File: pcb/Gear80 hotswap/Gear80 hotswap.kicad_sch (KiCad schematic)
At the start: 206 parts, among them J3 Conn_01x04, U1 RP2040, U3 W25Q128JVSIQ, U4 XC6206P332MR, Y1 X322512MSB4SI

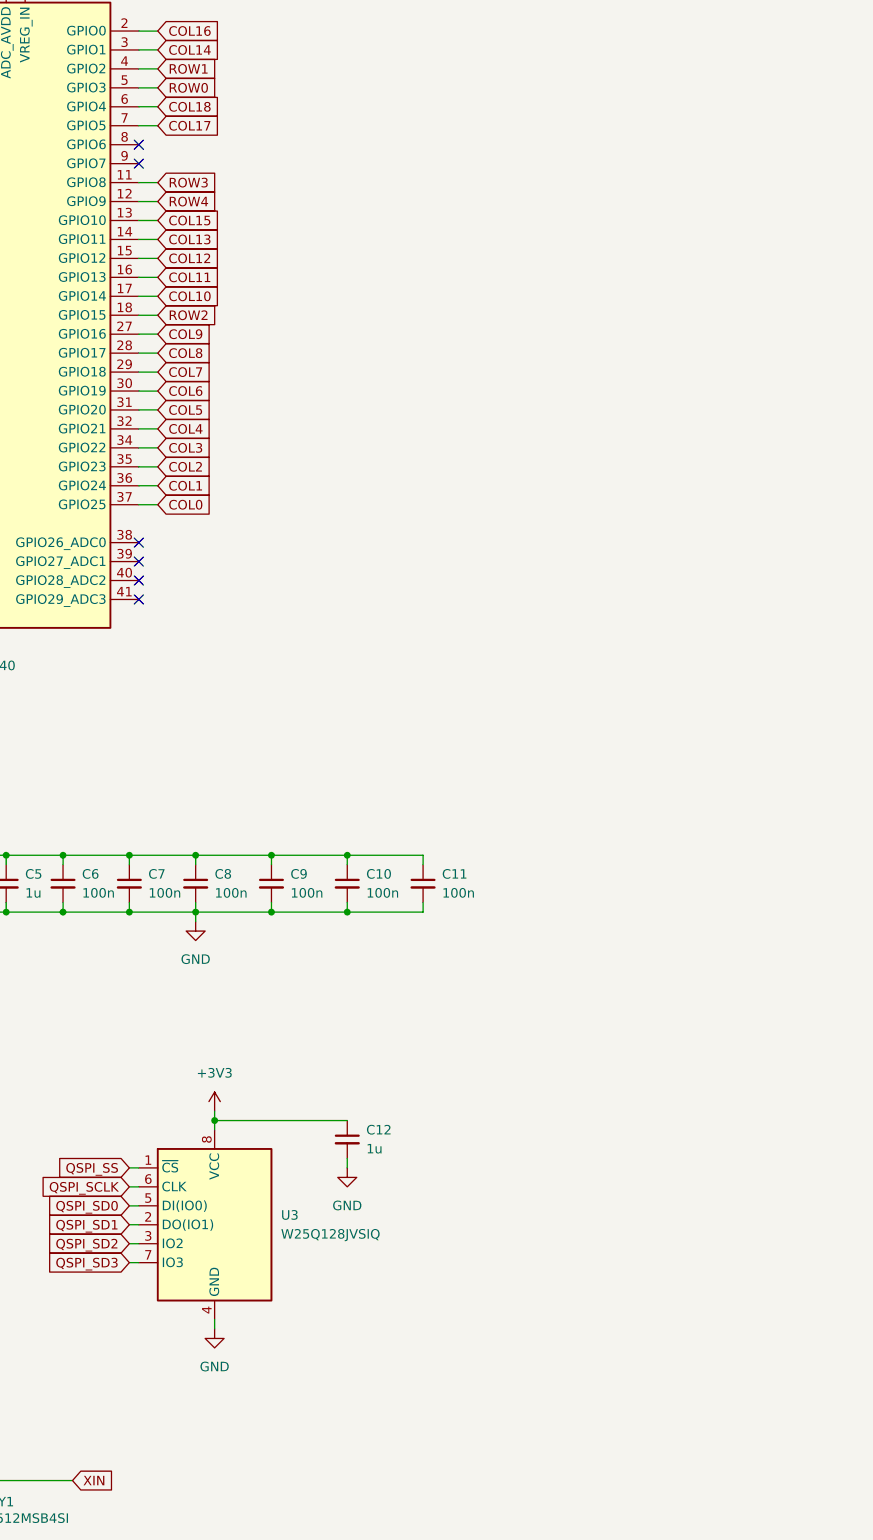
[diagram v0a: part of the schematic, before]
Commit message: Add files via upload
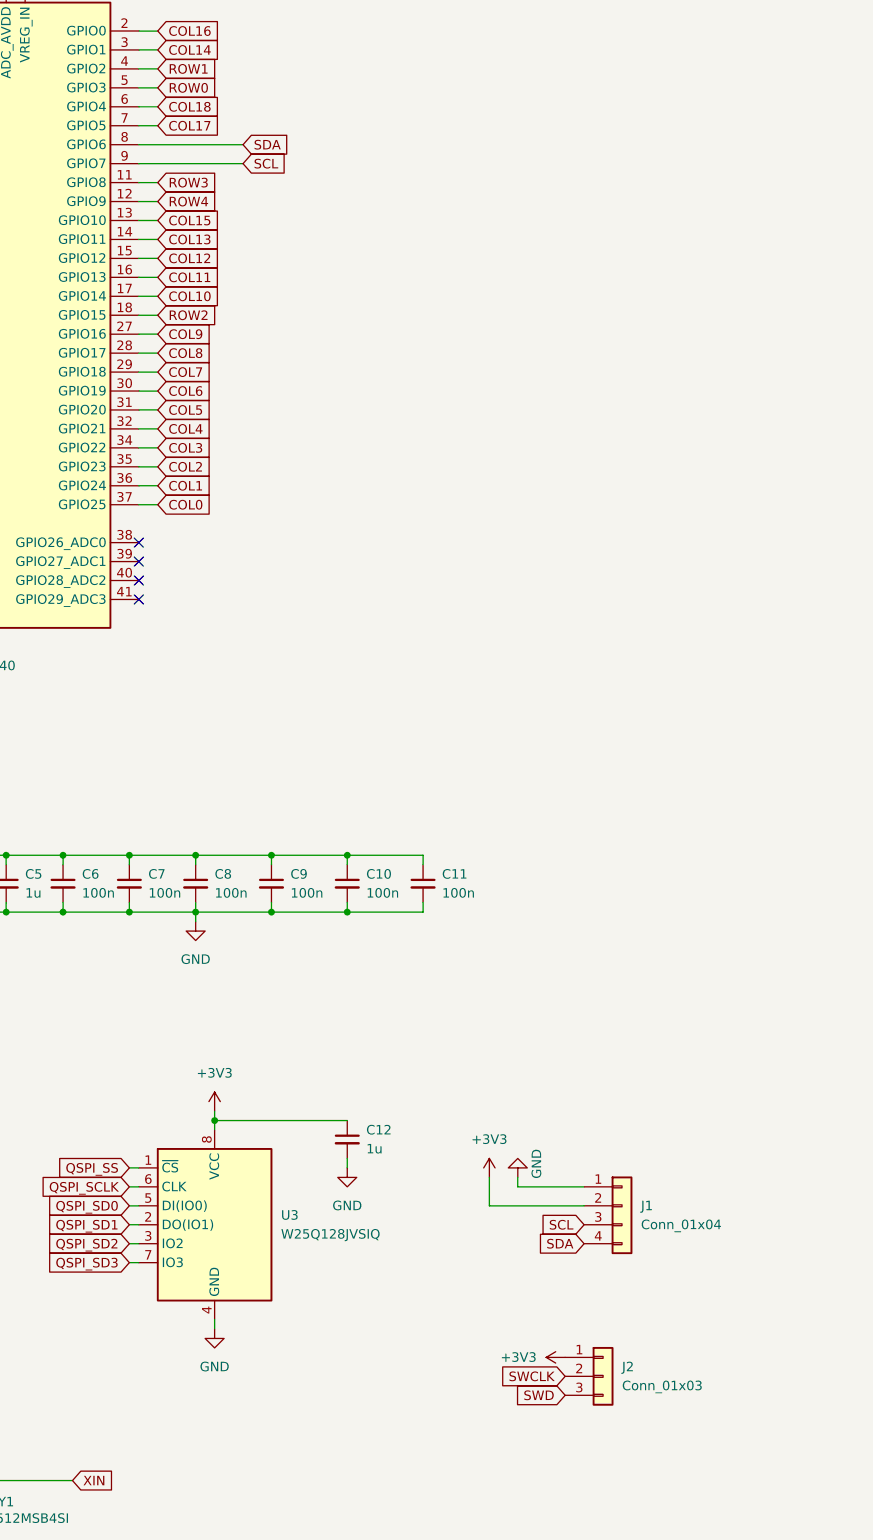
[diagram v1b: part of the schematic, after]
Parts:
- added J1: Conn_01x04, Connector_PinHeader_2.54mm:PinHeader_1x04_P2.54mm_Vertical, symbol Connector_Generic:Conn_01x04
- added J2: Conn_01x03, Connector_PinHeader_2.54mm:PinHeader_1x03_P2.54mm_Vertical, symbol Connector_Generic:Conn_01x03
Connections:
- net +3V3: now also J1.2 (Pin_2), J2.1 (Pin_1)
- net GND: now also J1.1 (Pin_1)
- net SWCLK: now also J2.2 (Pin_2)
- net SWD: now also J2.3 (Pin_3)
- net SDA: now reaches U1.8 (GPIO6)
- net SDA: now also J1.4 (Pin_4)
- net SCL: now reaches U1.9 (GPIO7)
- net SCL: now also J1.3 (Pin_3)
- no-connect marks 6 -> 4
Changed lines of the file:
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@@
   (no_connect (at 90.17 102.87))
   (no_connect (at 90.17 105.41))
-  (no_connect (at 90.17 49.53))
   (no_connect (at 90.17 107.95))
-  (no_connect (at 90.17 46.99))
   (no_connect (at 90.17 100.33))
   (wire (pts (xy 227.33 58.42) (xy 227.33 59.69))
@@
     (stroke (width 0) (type default))
   )
+  (wire (pts (xy 140.97 186.69) (xy 149.86 186.69))
+    (stroke (width 0) (type default))
+  )
   (wire (pts (xy 54.61 264.16) (xy 54.61 265.43))
     (stroke (width 0) (type default))
@@
     (stroke (width 0) (type default))
   )
+  (wire (pts (xy 137.16 189.23) (xy 137.16 185.42))
+    (stroke (width 0) (type default))
+  )
   (wire (pts (xy 327.66 64.77) (xy 342.9 64.77))
     (stroke (width 0) (type default))
@@
     (stroke (width 0) (type default))
   )
+  (wire (pts (xy 137.16 189.23) (xy 149.86 189.23))
+    (stroke (width 0) (type default))
+  )
   (wire (pts (xy 353.06 45.72) (xy 353.06 53.34))
     (stroke (width 0) (type default))
@@
     (stroke (width 0) (type default))
   )
+  (wire (pts (xy 104.14 46.99) (xy 90.17 46.99))
+    (stroke (width 0) (type default))
+  )
   (wire (pts (xy 227.33 64.77) (xy 269.24 64.77))
     (stroke (width 0) (type default))
@@
     (stroke (width 0) (type default))
   )
+  (wire (pts (xy 104.14 49.53) (xy 90.17 49.53))
+    (stroke (width 0) (type default))
+  )
   (wire (pts (xy 403.86 111.76) (xy 417.83 111.76))
     (stroke (width 0) (type default))
@@
     (stroke (width 0) (type default))
   )
+  (wire (pts (xy 140.97 185.42) (xy 140.97 186.69))
+    (stroke (width 0) (type default))
+  )
   (wire (pts (xy 398.78 124.46) (xy 398.78 147.32))
     (stroke (width 0) (type default))
@@
     )
   )
+  (global_label "SCL" (shape input) (at 104.14 49.53 0) (fields_autoplaced)
+    (effects (font (size 1.27 1.27)) (justify left))
+    (property "Intersheetrefs" "${INTERSHEET_REFS}" (at 110.6328 49.53 0)
+      (effects (font (size 1.27 1.27)) (justify left) hide)
+    )
+  )
   (global_label "QSPI_SS" (shape input) (at 55.88 278.13 0) (fields_autoplaced)
     (effects (font (size 1.27 1.27)) (justify left))
@@
     )
   )
+  (global_label "SDA" (shape input) (at 149.86 194.31 180) (fields_autoplaced)
+    (effects (font (size 1.27 1.27)) (justify right))
+    (property "Intersheetrefs" "${INTERSHEET_REFS}" (at 143.3067 194.31 0)
+      (effects (font (size 1.27 1.27)) (justify right) hide)
+    )
+  )
   (global_label "COL7" (shape input) (at 337.82 45.72 90) (fields_autoplaced)
     (effects (font (size 1.27 1.27)) (justify left))
@@
     )
   )
+  (global_label "SWD" (shape input) (at 147.32 214.63 180) (fields_autoplaced)
+    (effects (font (size 1.27 1.27)) (justify right))
+    (property "Intersheetrefs" "${INTERSHEET_REFS}" (at 140.4039 214.63 0)
+      (effects (font (size 1.27 1.27)) (justify right) hide)
+    )
+  )
   (global_label "COL0" (shape input) (at 92.71 95.25 0) (fields_autoplaced)
     (effects (font (size 1.27 1.27)) (justify left))
@@
     )
   )
+  (global_label "SWCLK" (shape input) (at 147.32 212.09 180) (fields_autoplaced)
+    (effects (font (size 1.27 1.27)) (justify right))
+    (property "Intersheetrefs" "${INTERSHEET_REFS}" (at 138.1058 212.09 0)
+      (effects (font (size 1.27 1.27)) (justify right) hide)
+    )
+  )
   (global_label "QSPI_SD1" (shape input) (at 88.9 191.77 180) (fields_autoplaced)
     (effects (font (size 1.27 1.27)) (justify right))
@@
     )
   )
+  (global_label "SDA" (shape input) (at 104.14 46.99 0) (fields_autoplaced)
+    (effects (font (size 1.27 1.27)) (justify left))
+    (property "Intersheetrefs" "${INTERSHEET_REFS}" (at 110.6933 46.99 0)
+      (effects (font (size 1.27 1.27)) (justify left) hide)
+    )
+  )
   (global_label "COL0" (shape input) (at 207.01 45.72 90) (fields_autoplaced)
     (effects (font (size 1.27 1.27)) (justify left))
@@
     )
   )
+  (global_label "SCL" (shape input) (at 149.86 191.77 180) (fields_autoplaced)
+    (effects (font (size 1.27 1.27)) (justify right))
+    (property "Intersheetrefs" "${INTERSHEET_REFS}" (at 143.3672 191.77 0)
+      (effects (font (size 1.27 1.27)) (justify right) hide)
+    )
+  )
   (global_label "XOUT" (shape input) (at 81.28 236.22 0) (fields_autoplaced)
     (effects (font (size 1.27 1.27)) (justify left))
@@
     )
   )
+  (symbol (lib_id "Connector_Generic:Conn_01x04") (at 154.94 189.23 0) (unit 1)
+    (in_bom yes) (on_board yes) (dnp no) (fields_autoplaced)
+    (property "Reference" "J1" (at 157.48 189.23 0)
+      (effects (font (size 1.27 1.27)) (justify left))
+    )
+    (property "Value" "Conn_01x04" (at 157.48 191.77 0)
+      (effects (font (size 1.27 1.27)) (justify left))
+    )
+    (property "Footprint" "Connector_PinHeader_2.54mm:PinHeader_1x04_P2.54mm_Vertical" (at 154.94 189.23 0)
+      (effects (font (size 1.27 1.27)) hide)
+    )
+    (property "Datasheet" "~" (at 154.94 189.23 0)
+      (effects (font (size 1.27 1.27)) hide)
+    )
+    (pin "1")
+    (pin "2")
+    (pin "3")
+    (pin "4")
+    (instances
+      (project "Gear80 hotswap"
+        (path "/3cbd346f-f2f7-49f7-a092-ced5397d72c6"
+          (reference "J1") (unit 1)
+        )
+      )
+    )
+  )
   (symbol (lib_id "power:GND") (at 118.11 184.15 0) (unit 1)
     (in_bom yes) (on_board yes) (dnp no) (fields_autoplaced)
@@
     )
   )
+  (symbol (lib_id "power:+3V3") (at 137.16 185.42 0) (unit 1)
+    (in_bom yes) (on_board yes) (dnp no) (fields_autoplaced)
+    (property "Reference" "#PWR08" (at 137.16 189.23 0)
+      (effects (font (size 1.27 1.27)) hide)
+    )
+    (property "Value" "+3V3" (at 137.16 180.34 0)
+      (effects (font (size 1.27 1.27)))
+    )
+    (property "Footprint" "" (at 137.16 185.42 0)
+      (effects (font (size 1.27 1.27)) hide)
+    )
+    (property "Datasheet" "" (at 137.16 185.42 0)
+      (effects (font (size 1.27 1.27)) hide)
+    )
+    (pin "1")
+    (instances
+      (project "Gear80 hotswap"
+        (path "/3cbd346f-f2f7-49f7-a092-ced5397d72c6"
+          (reference "#PWR08") (unit 1)
+        )
+      )
+      (project "gear"
+        (path "/b7ecd40f-fbd1-4363-aa36-fbfbff6aee59"
+          (reference "#PWR04") (unit 1)
+        )
+      )
+    )
+  )
   (symbol (lib_id "PCM_marbastlib-mx:MX_SW_HS") (at 209.55 127 0) (unit 1)
     (in_bom yes) (on_board yes) (dnp no) (fields_autoplaced)
@@
     )
   )
+  (symbol (lib_id "power:GND") (at 140.97 185.42 180) (unit 1)
+    (in_bom yes) (on_board yes) (dnp no)
+    (property "Reference" "#PWR09" (at 140.97 179.07 0)
+      (effects (font (size 1.27 1.27)) hide)
+    )
+    (property "Value" "GND" (at 143.51 181.61 90)
+      (effects (font (size 1.27 1.27)) (justify left))
+    )
+    (property "Footprint" "" (at 140.97 185.42 0)
+      (effects (font (size 1.27 1.27)) hide)
+    )
+    (property "Datasheet" "" (at 140.97 185.42 0)
+      (effects (font (size 1.27 1.27)) hide)
+    )
+    (pin "1")
+    (instances
+      (project "Gear80 hotswap"
+        (path "/3cbd346f-f2f7-49f7-a092-ced5397d72c6"
+          (reference "#PWR09") (unit 1)
+        )
+      )
+      (project "gear"
+        (path "/b7ecd40f-fbd1-4363-aa36-fbfbff6aee59"
+          (reference "#PWR017") (unit 1)
+        )
+      )
+    )
+  )
   (symbol (lib_id "PCM_marbastlib-mx:MX_SW_HS") (at 430.53 102.87 0) (unit 1)
     (in_bom yes) (on_board yes) (dnp no) (fields_autoplaced)
@@
     )
   )
+  (symbol (lib_id "power:+3V3") (at 147.32 209.55 90) (unit 1)
+    (in_bom yes) (on_board yes) (dnp no) (fields_autoplaced)
+    (property "Reference" "#PWR010" (at 151.13 209.55 0)
+      (effects (font (size 1.27 1.27)) hide)
+    )
+    (property "Value" "+3V3" (at 143.51 209.55 90)
+      (effects (font (size 1.27 1.27)) (justify left))
+    )
+    (property "Footprint" "" (at 147.32 209.55 0)
+      (effects (font (size 1.27 1.27)) hide)
+    )
+    (property "Datasheet" "" (at 147.32 209.55 0)
+      (effects (font (size 1.27 1.27)) hide)
+    )
+    (pin "1")
+    (instances
+      (project "Gear80 hotswap"
+        (path "/3cbd346f-f2f7-49f7-a092-ced5397d72c6"
+          (reference "#PWR010") (unit 1)
+        )
+      )
+      (project "gear"
+        (path "/b7ecd40f-fbd1-4363-aa36-fbfbff6aee59"
+          (reference "#PWR04") (unit 1)
+        )
+      )
+    )
+  )
   (symbol (lib_id "power:+3V3") (at 100.33 176.53 0) (unit 1)
     (in_bom yes) (on_board yes) (dnp no) (fields_autoplaced)
@@
         )
       )
+    )
+  )
+  (symbol (lib_id "Connector_Generic:Conn_01x03") (at 152.4 212.09 0) (unit 1)
+    (in_bom yes) (on_board yes) (dnp no) (fields_autoplaced)
+    (property "Reference" "J2" (at 154.94 210.82 0)
+      (effects (font (size 1.27 1.27)) (justify left))
+    )
+    (property "Value" "Conn_01x03" (at 154.94 213.36 0)
+      (effects (font (size 1.27 1.27)) (justify left))
+    )
+    (property "Footprint" "Connector_PinHeader_2.54mm:PinHeader_1x03_P2.54mm_Vertical" (at 152.4 212.09 0)
+      (effects (font (size 1.27 1.27)) hide)
+    )
+    (property "Datasheet" "~" (at 152.4 212.09 0)
+      (effects (font (size 1.27 1.27)) hide)
+    )
+    (pin "1")
+    (pin "2")
+    (pin "3")
+    (instances
+      (project "Gear80 hotswap"
+        (path "/3cbd346f-f2f7-49f7-a092-ced5397d72c6"
+          (reference "J2") (unit 1)
+        )
+      )
